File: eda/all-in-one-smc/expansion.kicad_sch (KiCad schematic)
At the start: 7 parts, among them J6 Expansion, U13 74HCT138

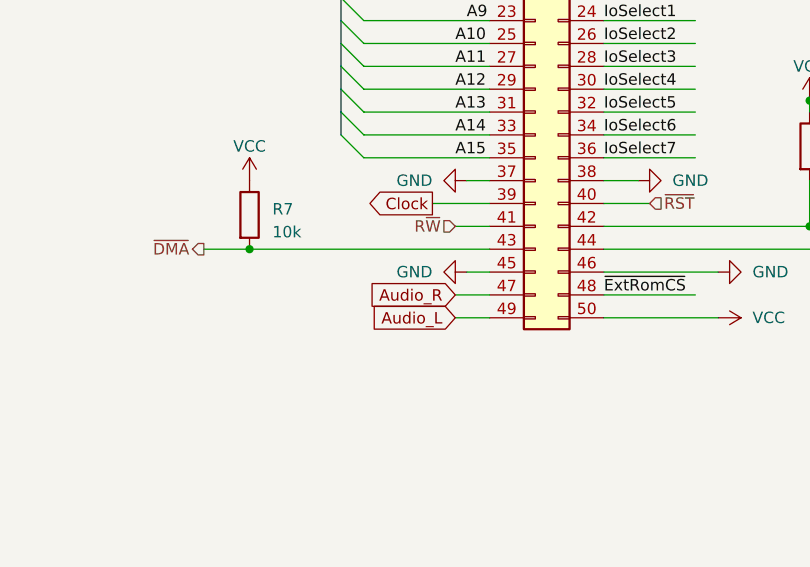
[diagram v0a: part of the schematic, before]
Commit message: wip
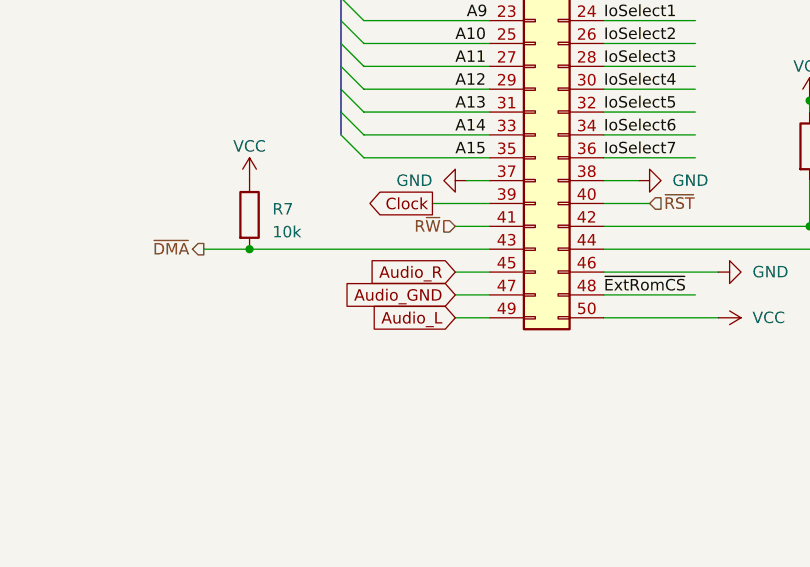
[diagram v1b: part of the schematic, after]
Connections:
- net Audio_R: now also J6.45 (Pin_45); no longer J6.47 (Pin_47)
- net GND: no longer J6.45 (Pin_45)
- new net Audio_GND: J6.47 (Pin_47)
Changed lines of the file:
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@@
 	(wire
 		(pts
-			(xy 130.81 96.52) (xy 133.35 96.52)
+			(xy 129.54 96.52) (xy 133.35 96.52)
 		)
 		(stroke
@@
 	(global_label "Audio_R"
 		(shape input)
-		(at 129.54 99.06 180)
+		(at 129.54 96.52 180)
 		(fields_autoplaced yes)
 		(effects
@@
 		)
 		(property "Intersheetrefs" "${INTERSHEET_REFS}"
-			(at 119.1768 99.06 0)
+			(at 119.1768 96.52 0)
 			(effects
 				(font
@@
 		(property "Intersheetrefs" "${INTERSHEET_REFS}"
 			(at 118.8933 88.9 0)
+			(effects
+				(font
+					(size 1.27 1.27)
+				)
+				(justify right)
+				(hide yes)
+			)
+		)
+	)
+	(global_label "Audio_GND"
+		(shape input)
+		(at 129.54 99.06 180)
+		(fields_autoplaced yes)
+		(effects
+			(font
+				(size 1.27 1.27)
+			)
+			(justify right)
+		)
+		(property "Intersheetrefs" "${INTERSHEET_REFS}"
+			(at 116.5763 99.06 0)
 			(effects
 				(font
@@
 					(unit 1)
 				)
-			)
-		)
-	)
-	(symbol
-		(lib_id "power:GND")
-		(at 130.81 96.52 270)
-		(unit 1)
-		(exclude_from_sim no)
-		(in_bom yes)
-		(on_board yes)
-		(dnp no)
-		(property "Reference" "#PWR053"
-			(at 124.46 96.52 0)
-			(effects
-				(font
-					(size 1.27 1.27)
-				)
-				(hide yes)
-			)
-		)
-		(property "Value" "GND"
-			(at 127 96.52 90)
-			(effects
-				(font
-					(size 1.27 1.27)
-				)
-				(justify right)
-			)
-		)
-		(property "Footprint" ""
-			(at 130.81 96.52 0)
-			(effects
-				(font
-					(size 1.27 1.27)
-				)
-				(hide yes)
-			)
-		)
-		(property "Datasheet" ""
-			(at 130.81 96.52 0)
-			(effects
-				(font
-					(size 1.27 1.27)
-				)
-				(hide yes)
-			)
-		)
-		(property "Description" ""
-			(at 130.81 96.52 0)
-			(effects
-				(font
-					(size 1.27 1.27)
-				)
-				(hide yes)
-			)
-		)
-		(pin "1"
-		)
-		(instances
-			(project "main-board"
-				(path "/2957ffac-6a43-4af7-8ab7-5cc1dbf2f2d7/e588fc5d-119a-48c2-8ca0-ace464ced7b8"
-					(reference "#PWR053")
-					(unit 1)
-				)
